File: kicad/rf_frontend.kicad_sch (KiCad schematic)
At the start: 6 parts, among them U10 LTC2311-16

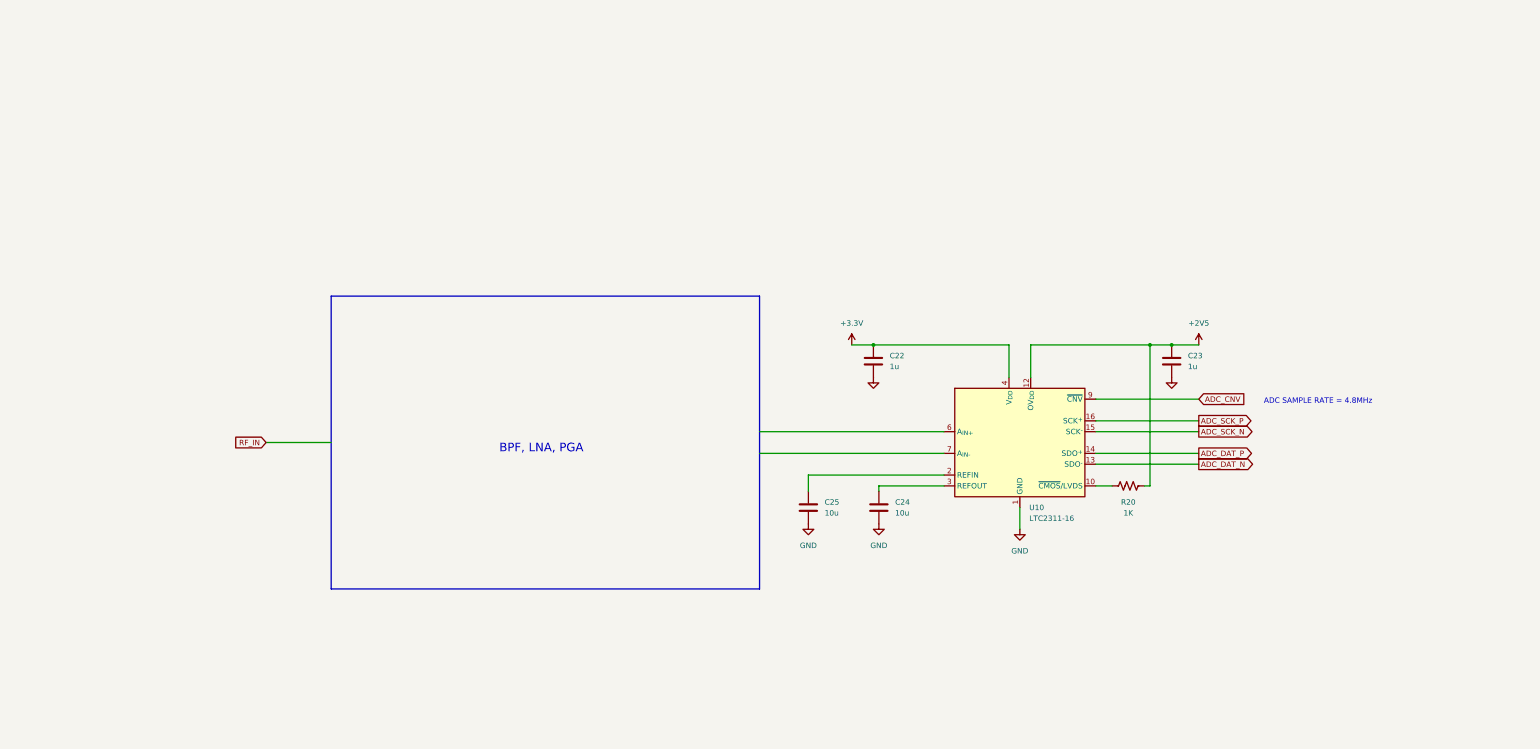
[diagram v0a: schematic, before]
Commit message: add some frontend stuff
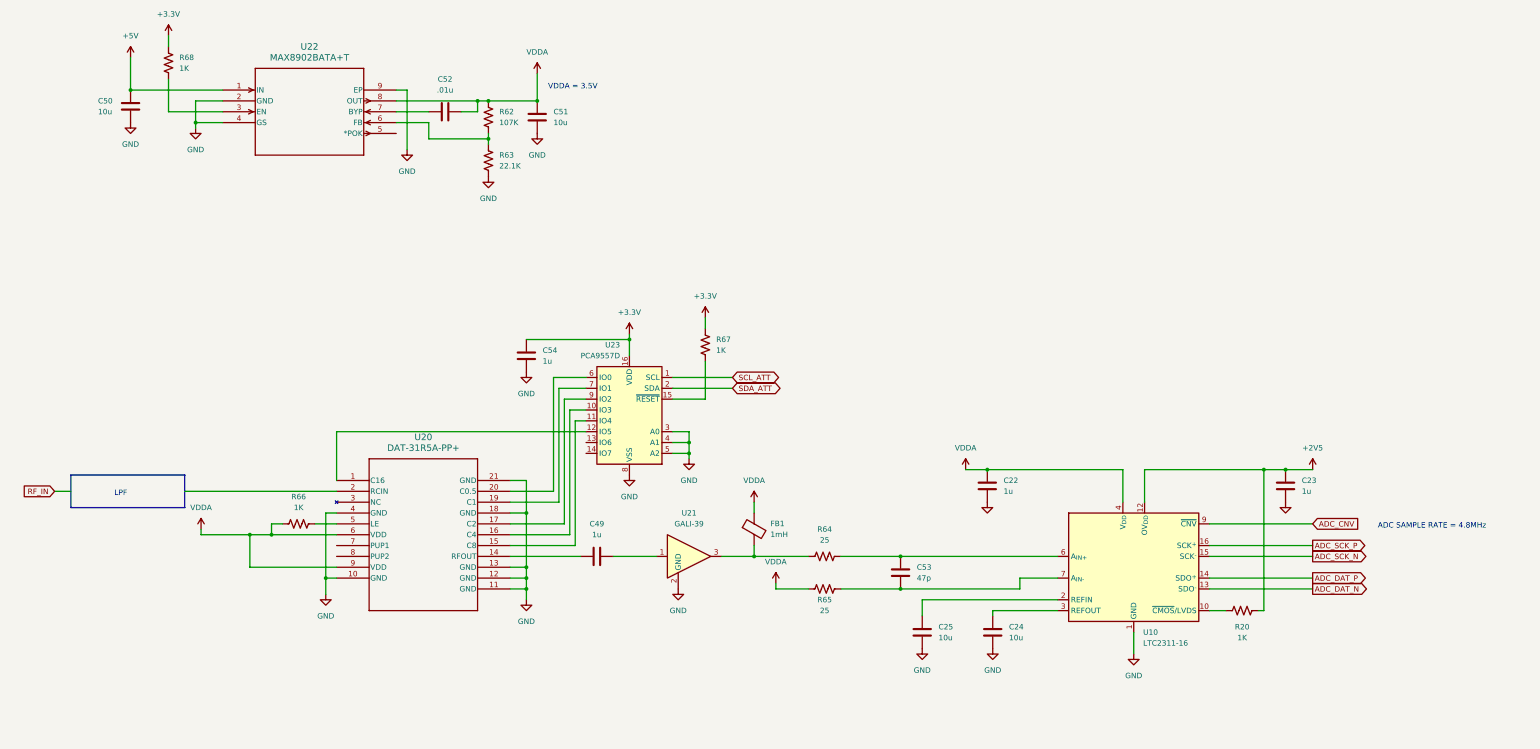
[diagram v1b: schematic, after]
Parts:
- added C49, C54: 1u, symbol Device:C
- added C50, C51: 10u, symbol Device:C
- added C52: .01u, symbol Device:C
- added C53: 47p, symbol Device:C
- added FB1: 1mH, symbol Device:FerriteBead
- added R62: 107K, symbol Device:R_US
- added R63: 22.1K, symbol Device:R_US
- added R64, R65: 25, symbol Device:R_US
- added R66, R67, R68: 1K, symbol Device:R_US
- added U20: DAT-31R5A-PP+, DG983-2_MNC, symbol bgelb_lib:DAT-31R5A-PP+
- added U21: GALI-39, Package_TO_SOT_SMD:SOT-89-3, symbol RF_Amplifier:GALI-39
- added U22: MAX8902BATA+T, 21-0168E_T822-1_MXM, symbol bgelb_lib:MAX8902BATA+T
- added U23: PCA9557D, Package_SO:SO-16_3.9x9.9mm_P1.27mm, symbol Interface_Expansion:PCA9557D
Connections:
- net +3.3V: now also C54.1, R67.1, R68.1, U23.16 (VDD); no longer C22.1, U10.4 (V_{DD})
- net GND: now also C50.2, C51.2, C54.2, R63.2, U20.10 (GND), U20.11 (GND), U20.12 (GND), U20.13 (GND), U20.18 (GND), U20.21 (GND), U20.4 (GND), U21.2 (GND), U22.2 (GND), U22.4 (GS), U22.9 (EP), U23.3 (A0), U23.4 (A1), U23.5 (A2), U23.8 (VSS)
- net at U10.6 (A_{IN+}): now also C53.1, R64.2
- net at U10.7 (A_{IN-}): now also C53.2, R65.2
- new net: C49.1, U20.14 (RFOUT)
- new net: C49.2, U21.1
- new net: R67.2, U23.15 (~{RESET})
- new net: FB1.2, R64.1, U21.3
- new net: R68.2, U22.3 (EN)
- new net: U20.16 (C4), U23.10 (IO3)
- new net: U20.15 (C8), U23.11 (IO4)
- new net: U20.1 (C16), U23.12 (IO5)
- new net: U20.20 (C0.5), U23.6 (IO0)
- new net: U20.19 (C1), U23.7 (IO1)
- new net: U20.17 (C2), U23.9 (IO2)
- new net: R62.2, R63.1, U22.6 (FB)
- new net: C52.1, U22.7 (BYP)
- new net: R66.1, U20.5 (LE)
- new net +5V: C50.1, U22.1 (IN)
- new net SCL_ATT: U23.1 (SCL)
- new net SDA_ATT: U23.2 (SDA)
- new net VDDA: C22.1, C51.1, C52.2, FB1.1, R62.1, R65.1, R66.2, U10.4 (V_{DD}), U20.6 (VDD), U20.9 (VDD), U22.8 (OUT)
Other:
- note added: "LPF"
- note added: "VDDA = 3.5V"
- note removed: "BPF, LNA, PGA"
- moved on the sheet: C22, C23, C24, C25, R20, U10

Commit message: frontend work
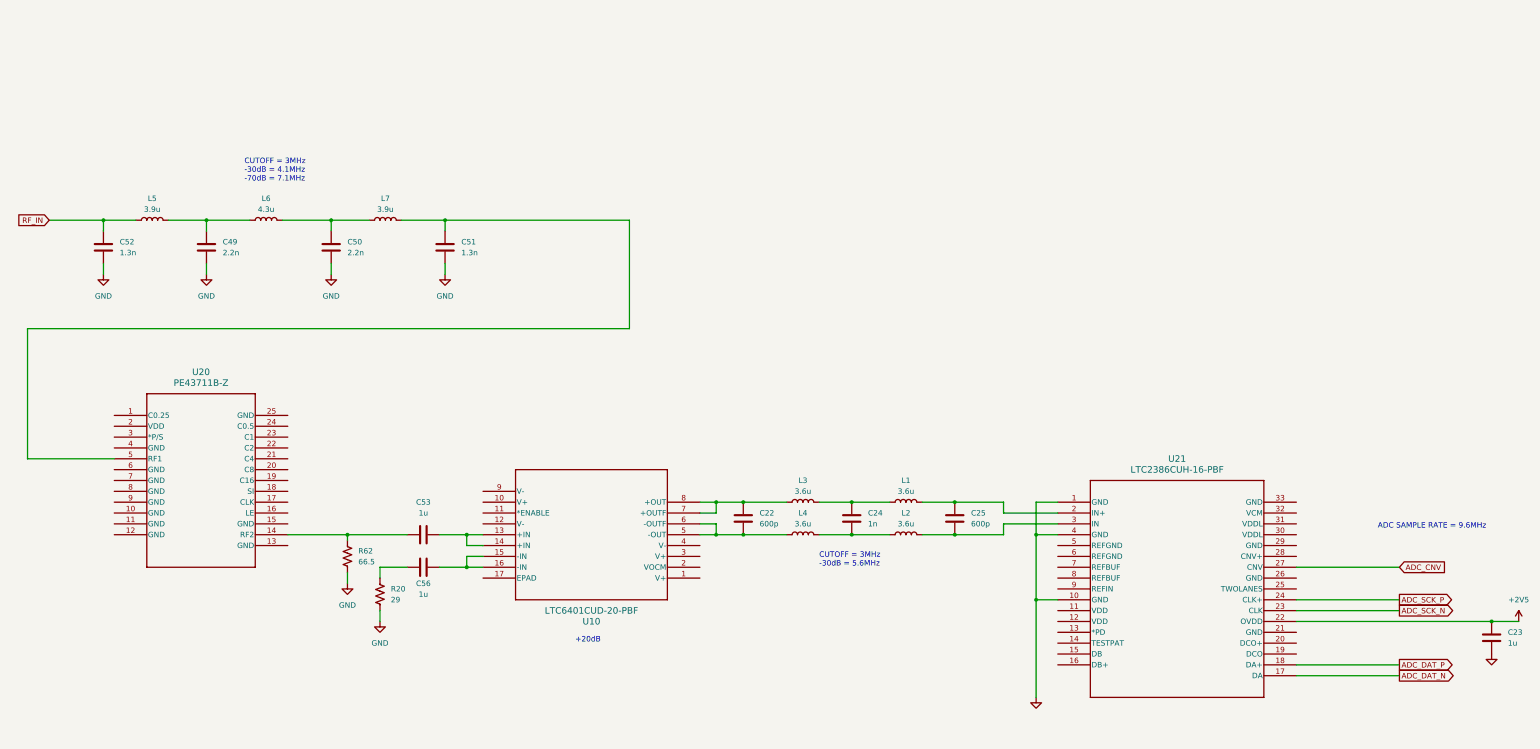
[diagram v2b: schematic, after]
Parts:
- removed C54: 1u, symbol Device:C
- removed FB1: 1mH, symbol Device:FerriteBead
- removed R63: 22.1K, symbol Device:R_US
- removed R64, R65: 25, symbol Device:R_US
- removed R66, R67, R68: 1K, symbol Device:R_US
- removed U10: LTC2311-16, Package_SO:MSOP-16-1EP_3x4.039mm_P0.5mm_EP1.651x2.845mm, symbol Analog_ADC:LTC2311-16
- removed U20: DAT-31R5A-PP+, DG983-2_MNC, symbol bgelb_lib:DAT-31R5A-PP+
- removed U21: GALI-39, Package_TO_SOT_SMD:SOT-89-3, symbol RF_Amplifier:GALI-39
- removed U22: MAX8902BATA+T, 21-0168E_T822-1_MXM, symbol bgelb_lib:MAX8902BATA+T
- removed U23: PCA9557D, Package_SO:SO-16_3.9x9.9mm_P1.27mm, symbol Interface_Expansion:PCA9557D
- added C56: 1u, symbol Device:C
- added L1, L2, L3, L4: 3.6u, symbol Device:L
- added L5, L7: 3.9u, symbol Device:L
- added L6: 4.3u, symbol Device:L
- added U10: LTC6401CUD-20-PBF, QFN-16_UD_LIT, symbol bgelb_lib:LTC6401CUD-20-PBF
- added U20: PE43711B-Z, QFN24_4X4_PSM, symbol bgelb_lib:PE43711B-Z
- added U21: LTC2386CUH-16-PBF, UH_32_ADI, symbol bgelb_lib:LTC2386CUH-16-PBF
- C22: value 1u -> 600p
- C24: value 10u -> 1n
- C25: value 10u -> 600p
- C49: value 1u -> 2.2n
- C50: value 10u -> 2.2n
- C51: value 10u -> 1.3n
- C52: value .01u -> 1.3n
- C53: value 47p -> 1u
- R20: value 1K -> 29
- R62: value 107K -> 66.5
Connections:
- net +2V5: now also U21.22 (OVDD); no longer R20.2
- net ADC_CNV: now also U21.27 (CNV)
- net ADC_DAT_N: now also U21.17 (DA)
- net ADC_DAT_P: now also U21.18 (DA+)
- net ADC_SCK_N: now also U21.23 (CLK)
- net ADC_SCK_P: now also U21.24 (CLK+)
- net GND: now also C49.2, C52.2, R20.2, R62.2, U21.1 (GND), U21.10 (GND), U21.4 (GND); no longer C22.2, C24.2, C25.2
- net RF_IN: now also C52.1, L5.1
- net at C25.1: now also L1.2, U21.2 (IN+)
- net at C53.2: now also U10.13 (+IN), U10.14 (+IN)
- net at C49.1: now also L5.2, L6.1
- net at C53.1: now also R62.1, U20.14 (RF2)
- net at C24.1: now also L1.1, L3.2
- net at R20.1: now also C56.1
- net +5V: no longer names the net of C50.1
- net +5V: now also L6.2, L7.1
- removed net VDDA: C22.1, C51.1, C52.2, R62.1
- new net: C56.2, U10.15 (-IN), U10.16 (-IN)
- new net: C22.2, L4.1, U10.5 (-OUT), U10.6 (-OUTF)
- new net: C22.1, L3.1, U10.7 (+OUTF), U10.8 (+OUT)
- new net: C24.2, L2.1, L4.2
- new net: C51.1, L7.2, U20.5 (RF1)
- new net: C25.2, L2.2, U21.3 (IN)
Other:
- note added: "+20dB"
- note added: "ADC SAMPLE RATE = 9.6MHz"
- note added: "CUTOFF = 3MHz -30dB = 4.1MHz -70dB = 7.1MHz"
- note added: "CUTOFF = 3MHz -30dB = 5.6MHz"
- note removed: "ADC SAMPLE RATE = 4.8MHz"
- note removed: "LPF"
- note removed: "VDDA = 3.5V"
- moved on the sheet: C23

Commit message: power and frontend updates
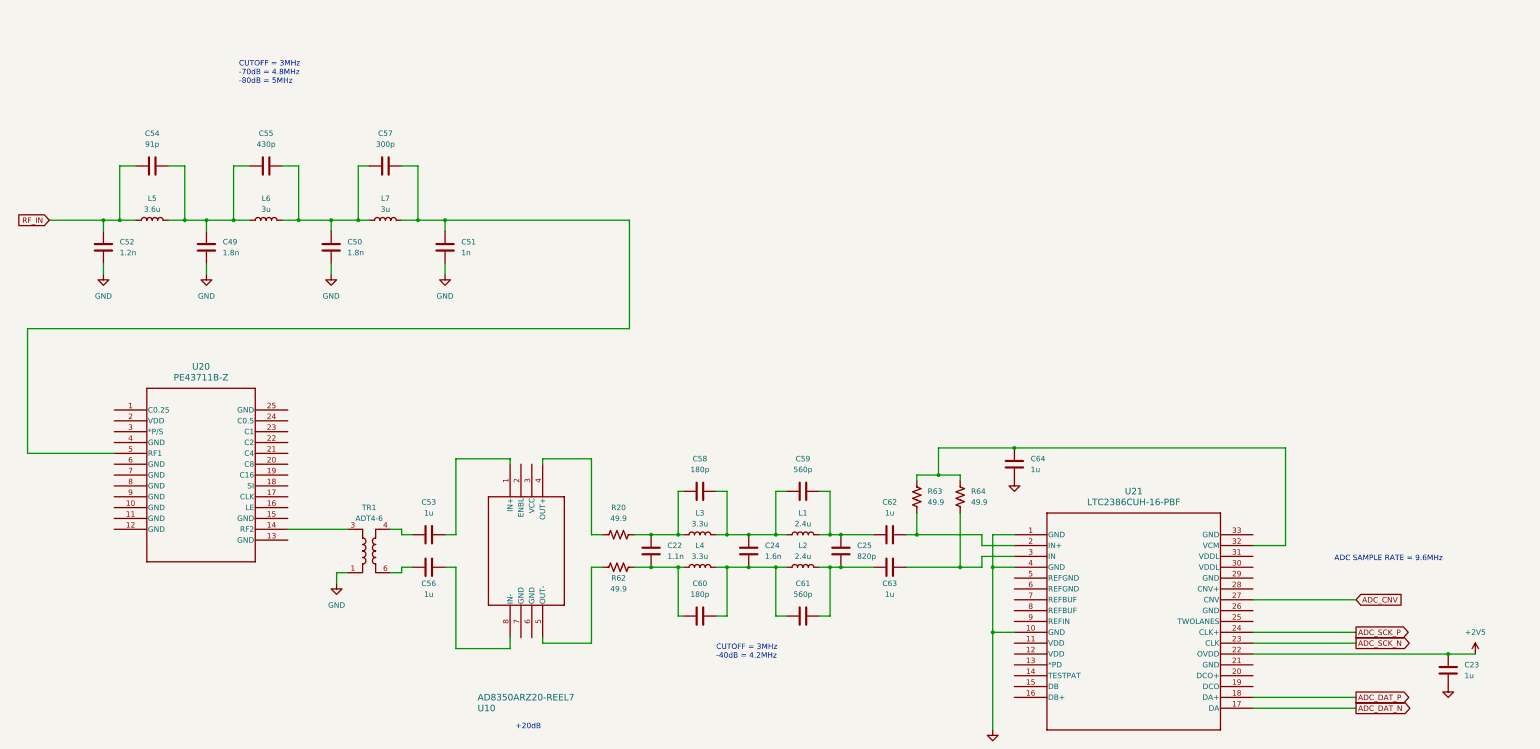
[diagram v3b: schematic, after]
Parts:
- removed U10: LTC6401CUD-20-PBF, QFN-16_UD_LIT, symbol bgelb_lib:LTC6401CUD-20-PBF
- added C54: 91p, symbol Device:C
- added C55: 430p, symbol Device:C
- added C57: 300p, symbol Device:C
- added C58, C60: 180p, symbol Device:C
- added C59, C61: 560p, symbol Device:C
- added C62, C63, C64: 1u, symbol Device:C
- added R63, R64: 49.9, symbol Device:R_US
- added TR1: ADT4-6, RF_Mini-Circuits:Mini-Circuits_CD637_H5.23mm, symbol Transformer:ADT4-6
- added U10: AD8350ARZ20-REEL7, R_8_ADI, symbol bgelb_lib:AD8350ARZ20-REEL7
- C22: value 600p -> 1.1n
- C24: value 1n -> 1.6n
- C25: value 600p -> 820p
- C49, C50: value 2.2n -> 1.8n
- C51: value 1.3n -> 1n
- C52: value 1.3n -> 1.2n
- L1, L2: value 3.6u -> 2.4u
- L3, L4: value 3.6u -> 3.3u
- L5: value 3.9u -> 3.6u
- L6: value 4.3u -> 3u
- L7: value 3.9u -> 3u
- R20: value 29 -> 49.9
- R62: value 66.5 -> 49.9
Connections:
- net GND: now also C64.2, TR1.1; no longer R20.2, R62.2
- net RF_IN: now also C54.1
- net at C53.2: now also U10.1 (IN+)
- net at C56.2: now also U10.8 (IN-)
- net at C22.2, L4.1: now also R62.2, C60.1
- net at C22.1, L3.1: now also R20.2, C58.1
- net at C24.2, L2.1, L4.2: now also C60.2, C61.1
- net at C50.1, L6.2, L7.1: now also C55.2, C57.1
- net at C51.1, L7.2, U20.5 (RF1): now also C57.2
- net at C25.1, L1.2: now also C59.2, C62.1; no longer U21.2 (IN+)
- net at C25.2, L2.2: now also C61.2, C63.1; no longer U21.3 (IN)
- net at U21.32 (VCM): now also C64.1, R63.1, R64.1
- net at C56.1: now also TR1.6; no longer R20.1
- net at C24.1, L1.1, L3.2: now also C58.2, C59.1
- net at C49.1, L5.2, L6.1: now also C54.2, C55.1
- new net: C62.2, R63.2, U21.2 (IN+)
- new net: C63.2, R64.2, U21.3 (IN)
- new net: R20.1, U10.4 (OUT+)
- new net: C53.1, TR1.4
- new net: TR1.3, U20.14 (RF2)
- new net: R62.1, U10.5 (OUT-)
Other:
- note added: "CUTOFF = 3MHz -40dB = 4.2MHz"
- note added: "CUTOFF = 3MHz -70dB = 4.8MHz -80dB = 5MHz"
- note removed: "CUTOFF = 3MHz -30dB = 4.1MHz -70dB = 7.1MHz"
- note removed: "CUTOFF = 3MHz -30dB = 5.6MHz"
- moved on the sheet: C22, C23, C24, C25, C53, C56, L1, L2, L3, L4, U20, U21
